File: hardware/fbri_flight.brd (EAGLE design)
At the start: 36 parts, among them U1 SAM_D20E, U2 SI4060, U3 MAX1947, U4 ANTENOVA_GPS_M10382, U5 S25FS-S

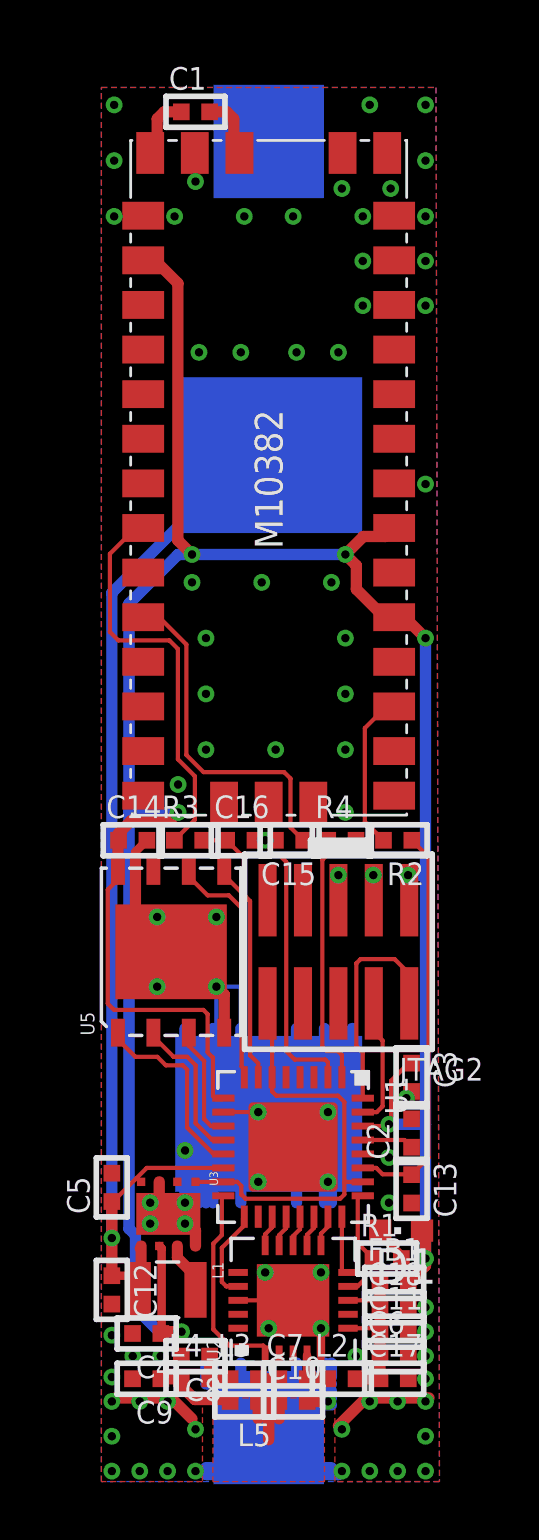
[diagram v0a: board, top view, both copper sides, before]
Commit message: Started work on development hardware
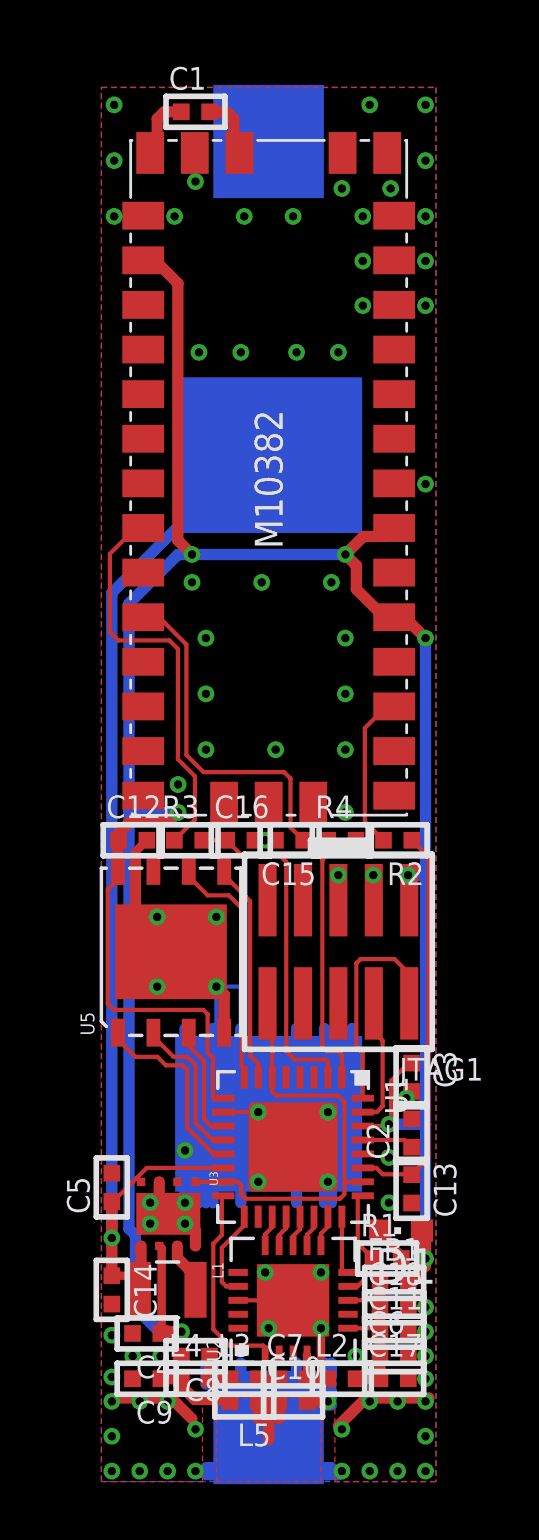
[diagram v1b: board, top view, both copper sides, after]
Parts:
- C1: value 100nF -> 15pF
- C12: value 100pF -> 100nF
- C14: value 100nF -> 100pF
- R2, R3, R4: value 1kΩ -> 100Ω
- moved C12 16.1 mm to (1.12, 23.0), turned to 0 degrees
- moved C14 16.1 mm to (0.38, 6.88), turned to 270 degrees
- renumbered JTAG2 to JTAG1, U$45 to J1
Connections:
- net 1.2V: now also C14.1; no longer C12.1
- net 1.8V: now also C12.1; no longer C14.1
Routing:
- net ANT: track 2.40 -> 4.40 mm
- net N$1: track 2.00 -> 0.00 mm
